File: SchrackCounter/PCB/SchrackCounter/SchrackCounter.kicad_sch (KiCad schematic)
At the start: 0 parts

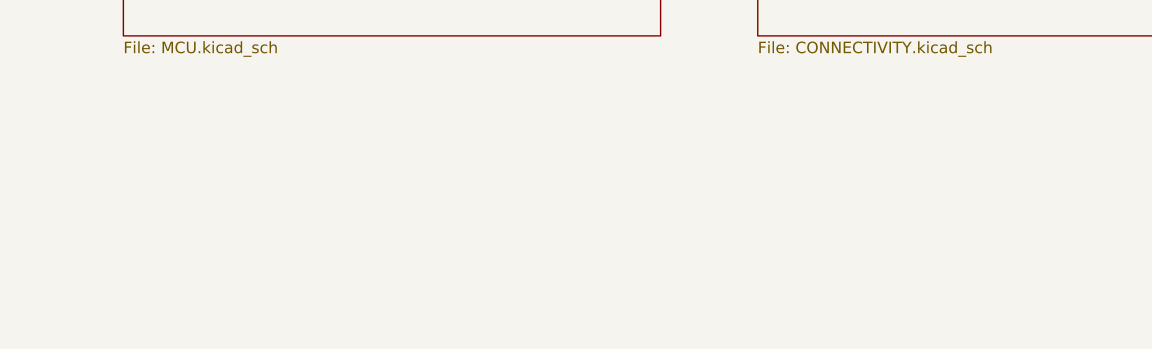
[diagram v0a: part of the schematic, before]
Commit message: fix?
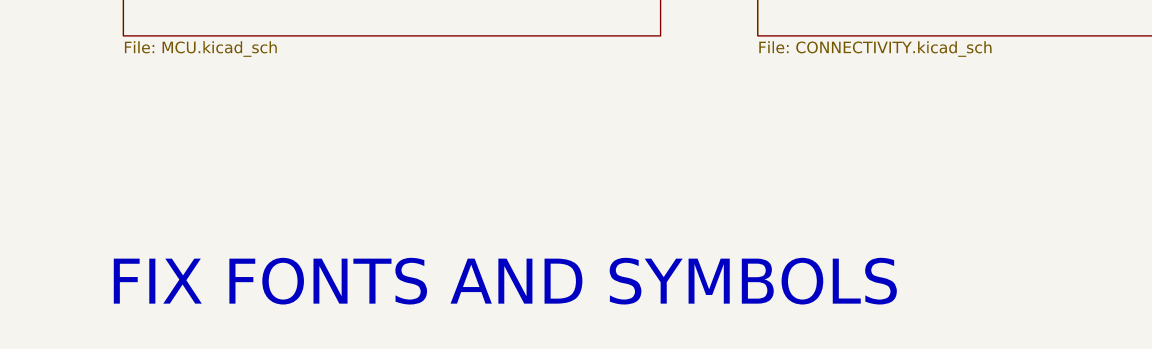
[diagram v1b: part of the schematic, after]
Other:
- note added: "FIX FONTS AND SYMBOLS"
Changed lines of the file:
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@@
 		(comment 1 "SAVVA POPOV")
+	)
+	(text "FIX FONTS AND SYMBOLS"
+		(exclude_from_sim no)
+		(at 86.106 173.736 0)
+		(effects
+			(font
+				(size 5 5)
+			)
+		)
 	)
 	(symbol
@@
 		)
 		(instances
-			(project ""
+			(project "SchrackCounter"
 				(path "/d96f2ffc-3f4c-4f71-b693-29f6b8c3245d"
 					(reference "#G1")
